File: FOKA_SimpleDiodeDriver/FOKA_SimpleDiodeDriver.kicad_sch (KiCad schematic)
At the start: 29 parts, among them J1 IN, J2 Conn_01x02, Q2 NMOS, U1 AZ431L, U2 ADA4891-1

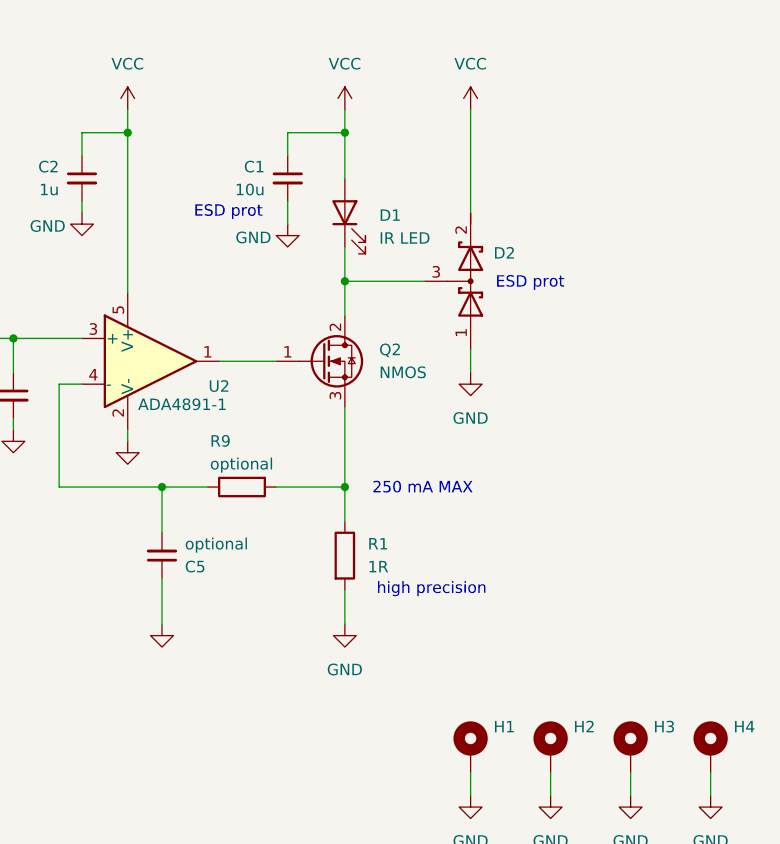
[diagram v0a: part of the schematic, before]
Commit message: RezystorDoBramki
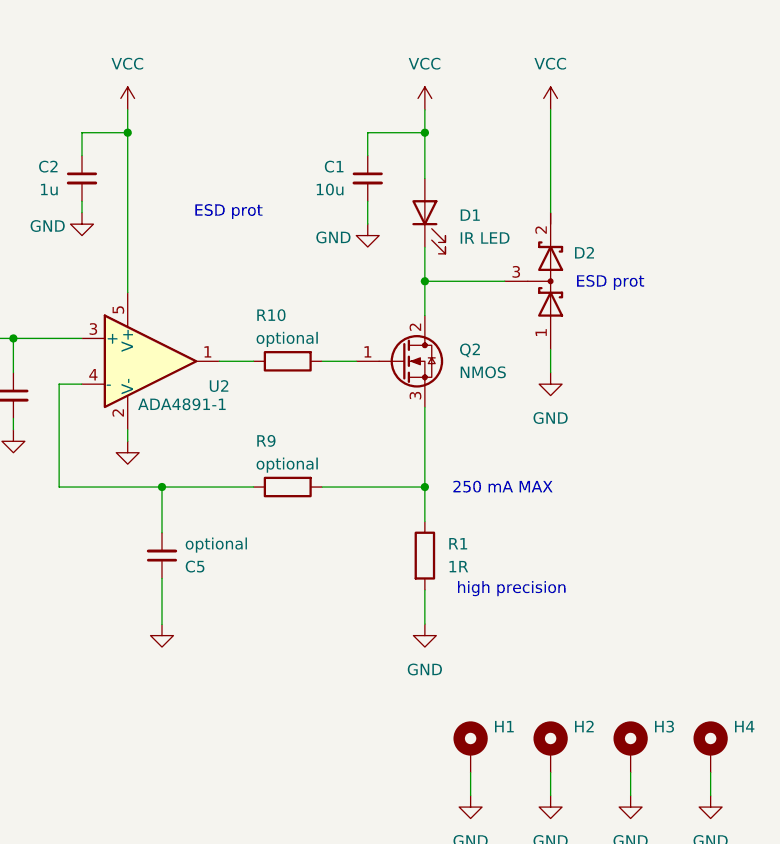
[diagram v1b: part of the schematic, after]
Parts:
- added R10: optional, Capacitor_SMD:C_0402_1005Metric, symbol Device:R
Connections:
- net at Q2.1 (G): now also R10.2; no longer U2.1
- new net: R10.1, U2.1
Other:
- moved on the sheet: C1, D1, D2, Q2, R1, R9
